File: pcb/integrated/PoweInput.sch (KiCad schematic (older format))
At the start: 28 parts, among them J8001 Conn_01x03_Female, Q8001 Q_NMOS_GDS, Q8002 2N7002, Q8003 Q_NMOS_GDS, U8001 VOM1271, U8002 UCC5350SB, U8003 ACS730

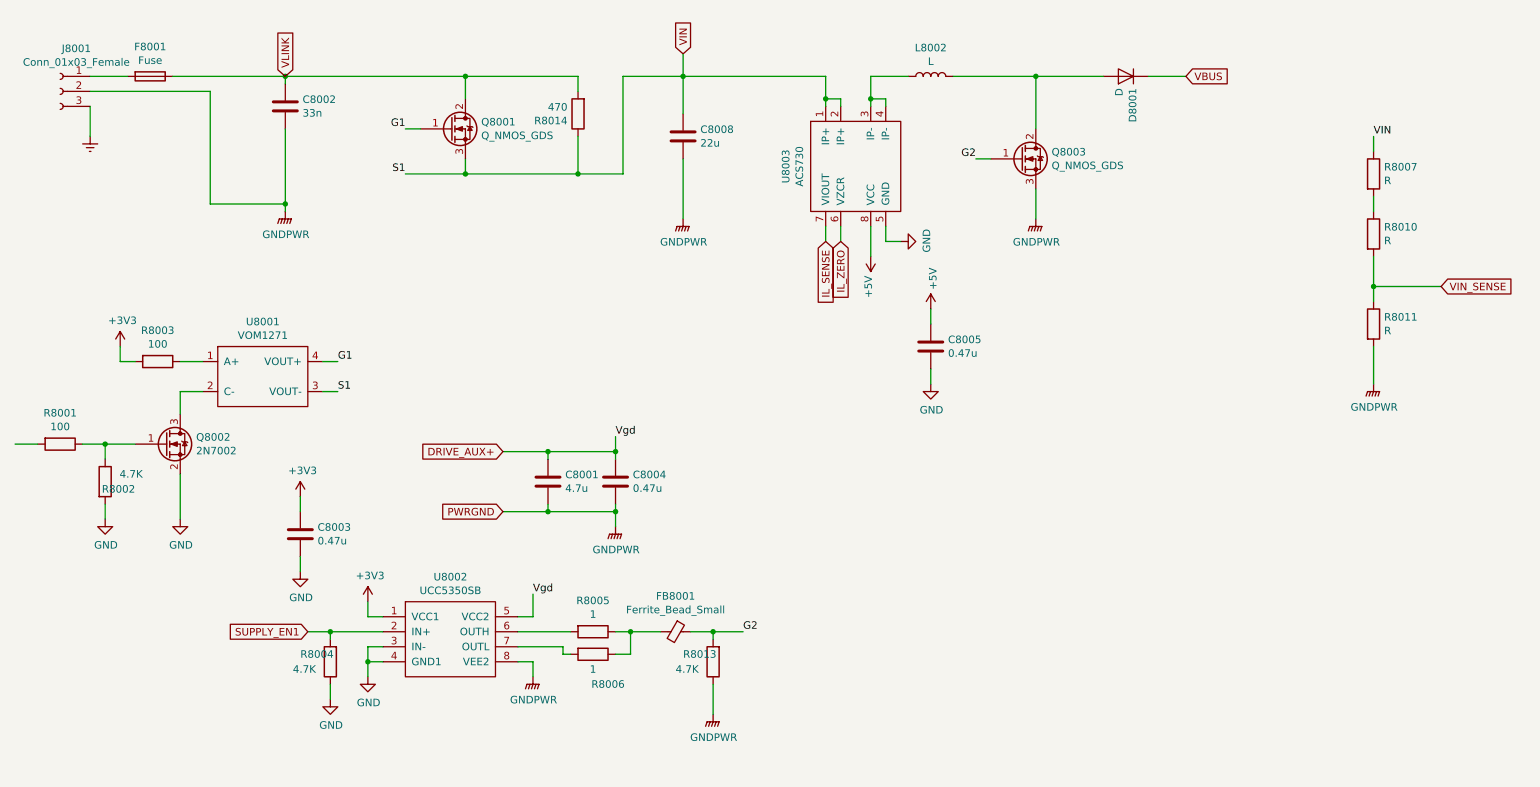
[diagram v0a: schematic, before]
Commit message: PCB routing finihsed, ready for design review
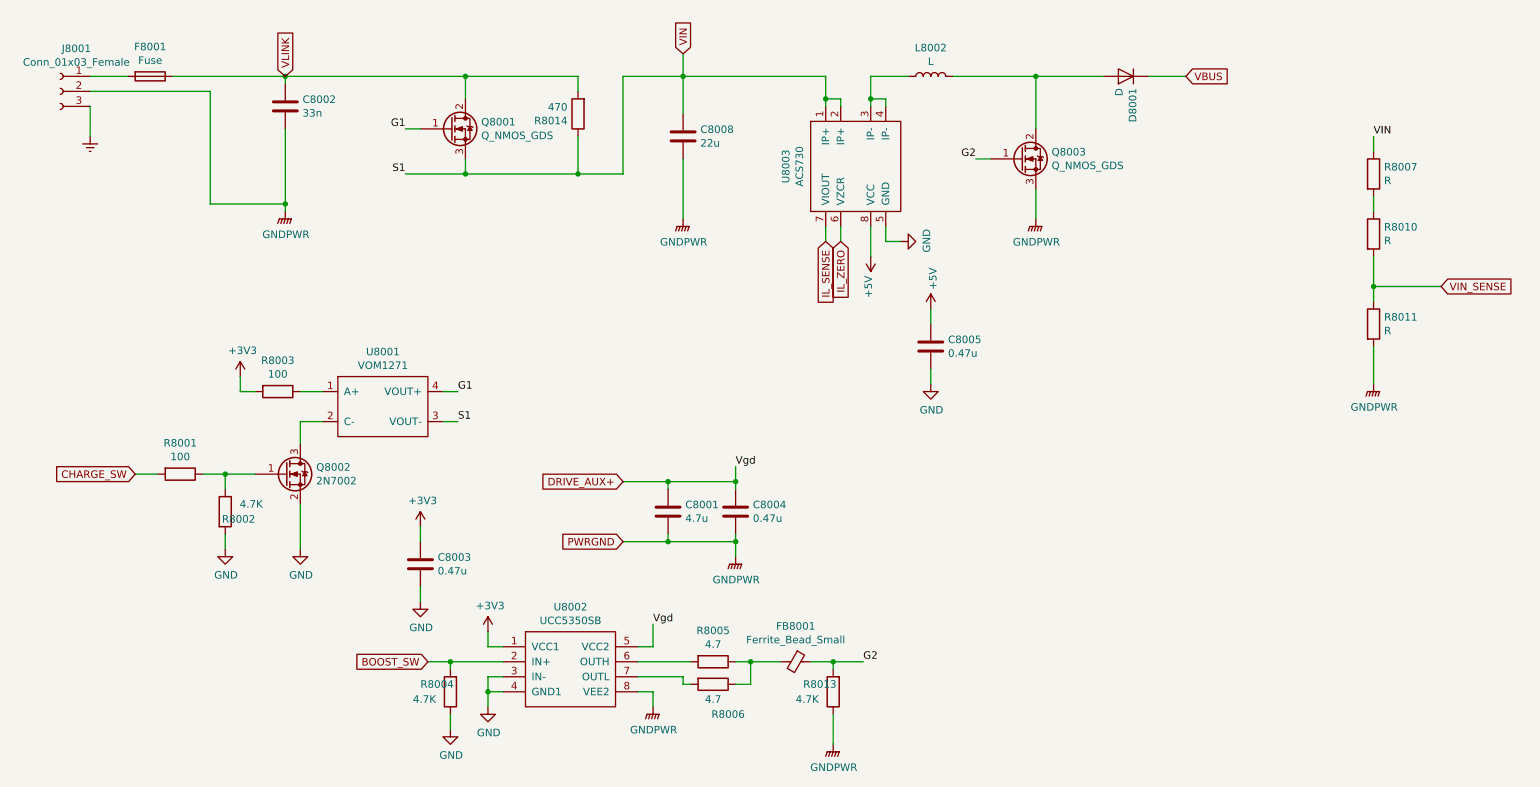
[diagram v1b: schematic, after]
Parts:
- R8005, R8006: value 1 -> 4.7
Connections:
- net CHARGE_SW: now reaches R8001.2
- net SUPPLY_EN1 renamed BOOST_SW
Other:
- moved on the sheet: C8001, C8003, C8004, FB8001, Q8002, R8001, R8002, R8003, R8004, R8005, R8006, R8013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
